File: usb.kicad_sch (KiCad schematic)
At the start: 44 parts, among them J27 USB_C_Receptacle_USB2.0_14P, J28 USB_C_Receptacle_USB2.0_14P, Q1 BSC098N10NS5, Q2 BSC098N10NS5, SW1 SW_DIP_x03, SW2 SW_DIP_x03, U2 CH224K, U20 LM5050-1, U21 LM5050-1, U22 CH224K

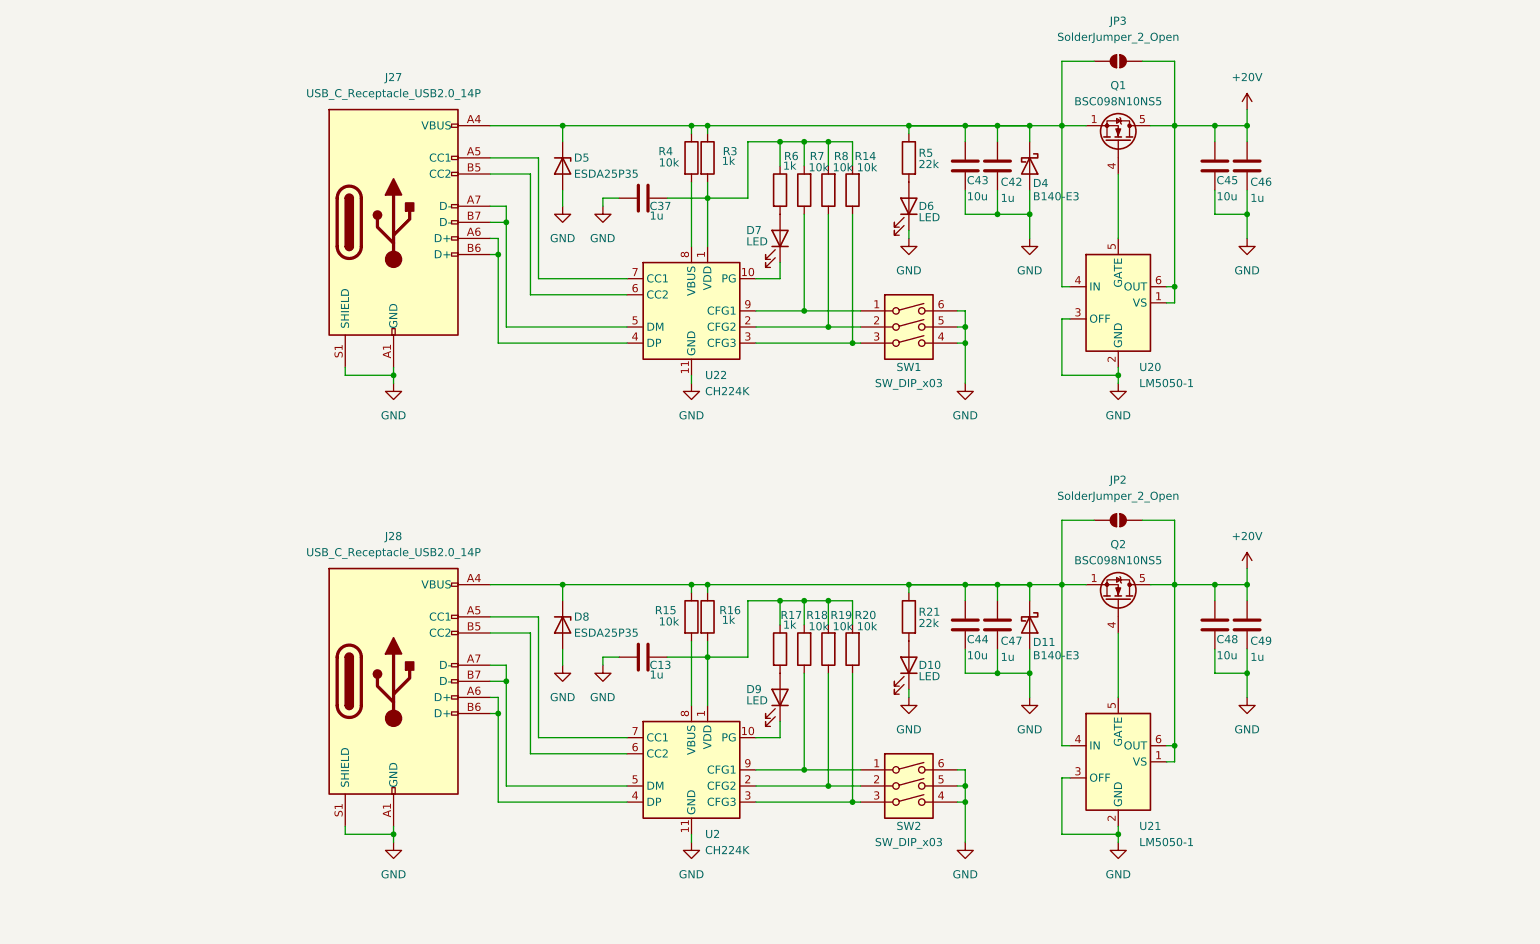
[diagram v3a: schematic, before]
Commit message: rewire
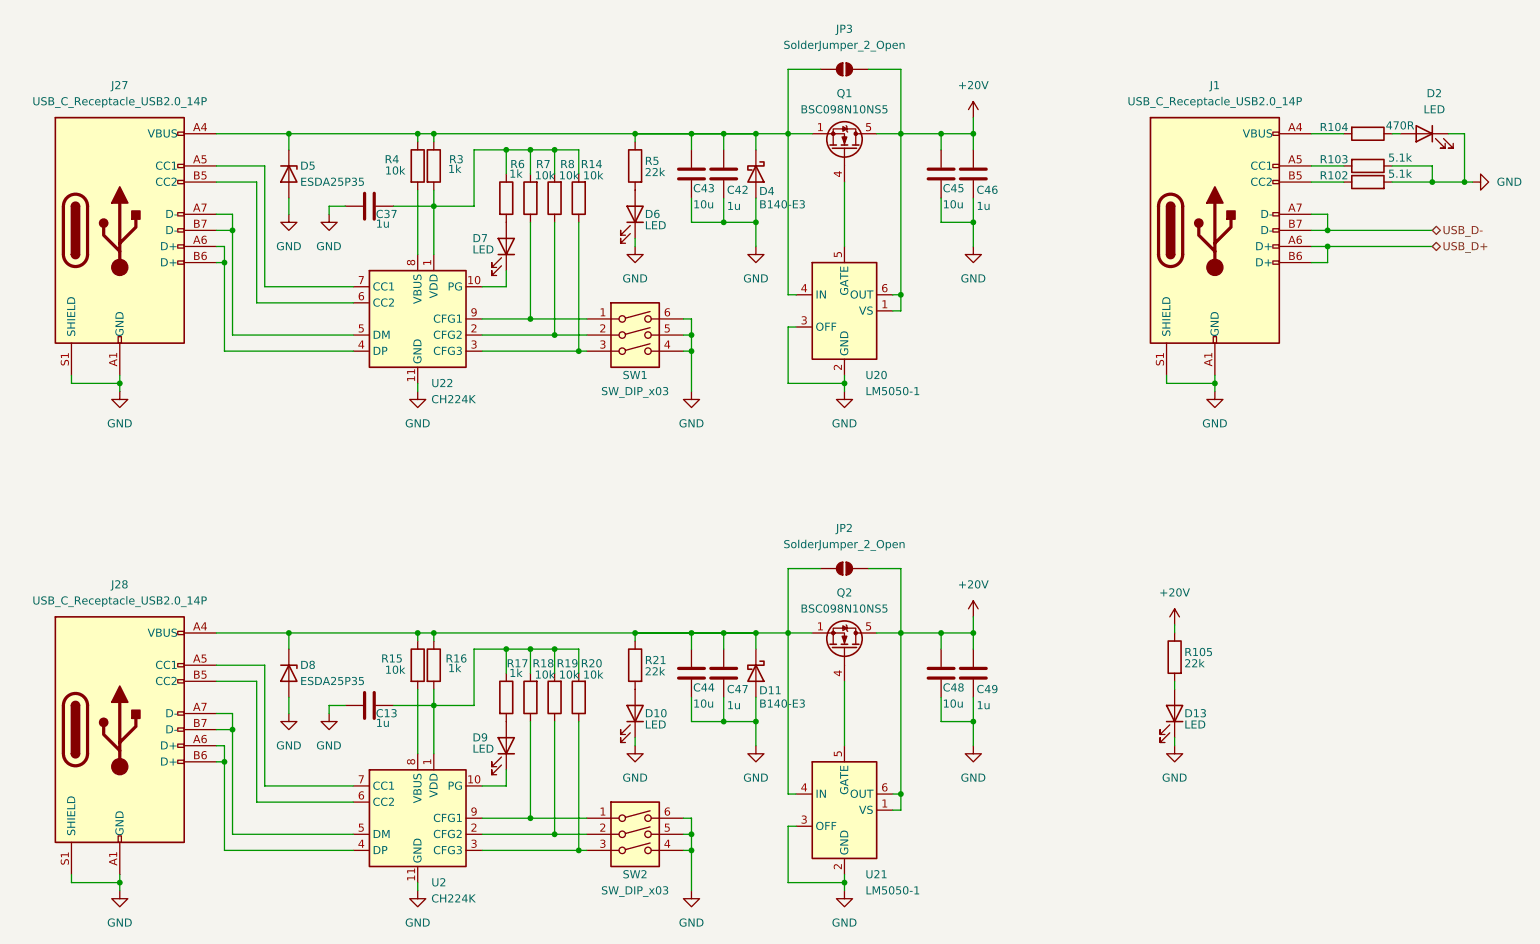
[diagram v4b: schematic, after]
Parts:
- added D13, D2: LED, symbol Device:LED
- added J1: USB_C_Receptacle_USB2.0_14P, symbol Connector:USB_C_Receptacle_USB2.0_14P
- added R102, R103: 5.1k, symbol Device:R
- added R104: 470R, symbol Device:R
- added R105: 22k, symbol Device:R
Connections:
- net +20V: now also R105.1
- net GND: now also D13.1 (K), D2.1 (K), J1.A1 (GND), J1.A12 (GND), J1.B1 (GND), J1.B12 (GND), J1.S1 (SHIELD), R102.2, R103.1
- new net: D2.2 (A), R104.1
- new net: J1.B5 (CC2), R102.1
- new net: D13.2 (A), R105.2
- new net: J1.A4 (VBUS), J1.A9 (VBUS), J1.B4 (VBUS), J1.B9 (VBUS), R104.2
- new net: J1.A5 (CC1), R103.2
- new net USB_D+: J1.A6 (D+), J1.B6 (D+)
- new net USB_D-: J1.A7 (D-), J1.B7 (D-)
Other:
- moved on the sheet: C13, C37, C42, C43, C44, C45, C46, C47, C48, C49, D10, D11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
